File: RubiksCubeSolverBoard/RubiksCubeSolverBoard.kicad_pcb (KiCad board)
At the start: 2 copper layers, 67 x 80.1 mm, 43 parts, among them J1 Power +12V, J10 MS3, J11 MS1, J12 Power +12V, J13 MS2, J14 MS3, J15 Motor2, J16 MS1, J17 MS2, J18 MS3, J19 Motor3, J2 Power +3.3V, J20 MS1, J21 MS2, J22 MS3, J23 Motor4, J24 MS1, J25 MS2, J26 MS3, J27 Motor5, J28 color sensor, J29 color sensor, J3 MS1, J4 BootOption, J6 SilentBoot, J7 Motor1, J8 Uart, J9 MS2, U1 ESP32-WROOM-32E

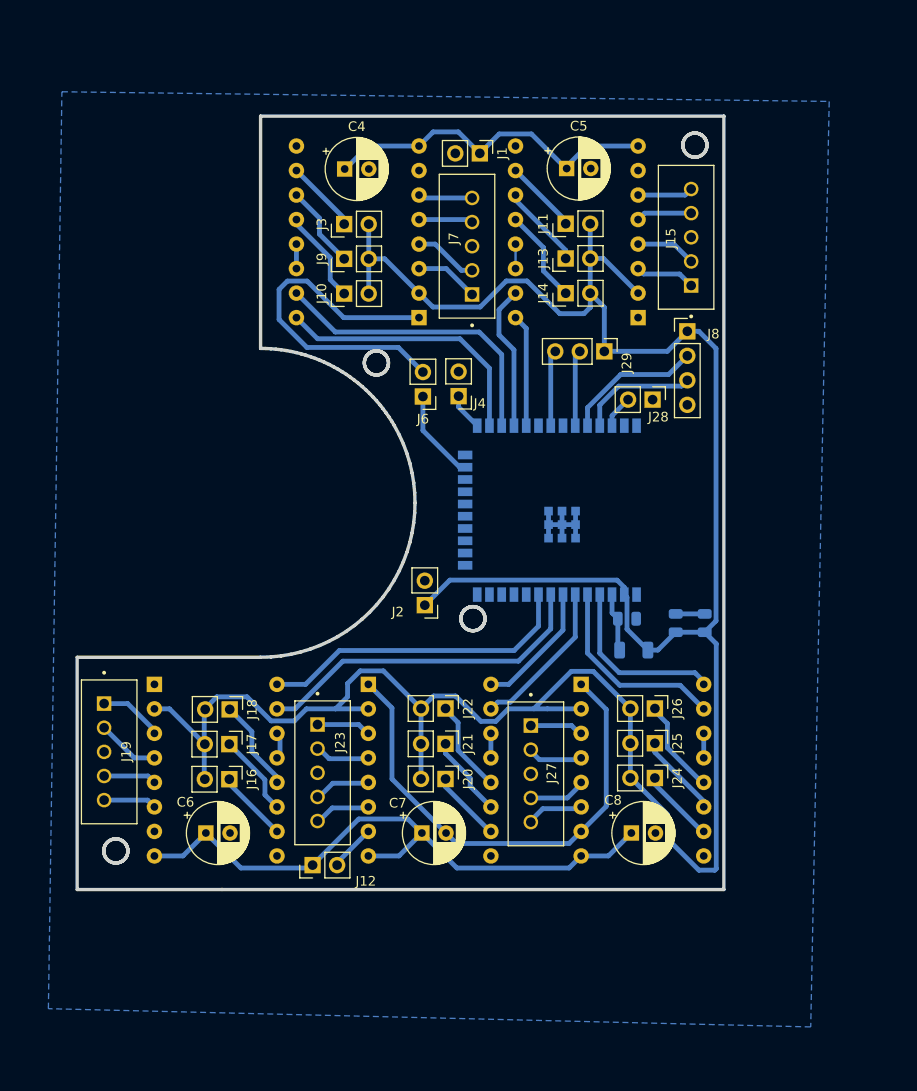
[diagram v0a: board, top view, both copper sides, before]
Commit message: 2 layer pcb
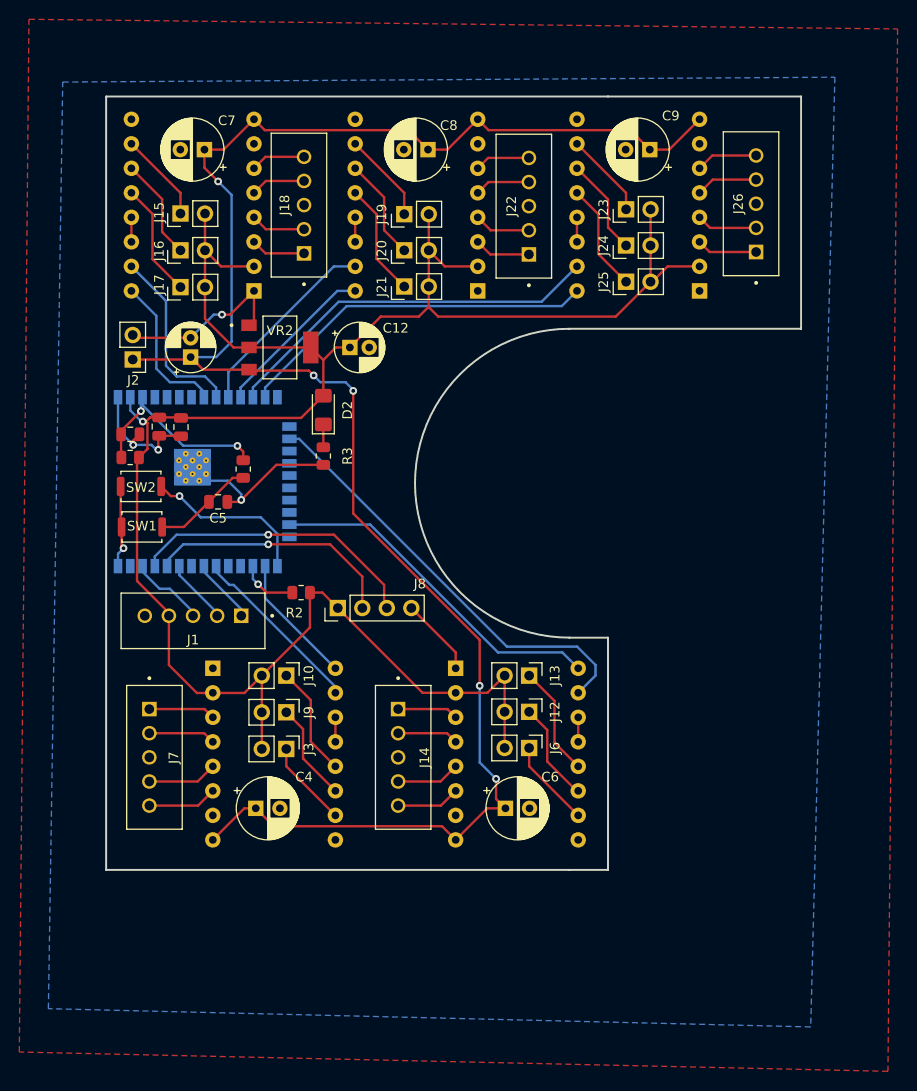
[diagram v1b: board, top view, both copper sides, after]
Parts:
- removed J11: MS1, Connector_PinHeader_2.54mm:PinHeader_1x02_P2.54mm_Vertical
- removed J27: Motor5, CustomParts:JST_B5B-XH-A_LF__SN_
- removed J28: color sensor, Connector_PinHeader_2.54mm:PinHeader_1x02_P2.54mm_Vertical
- removed J29: color sensor, Connector_PinHeader_2.54mm:PinHeader_1x03_P2.54mm_Vertical
- removed J4: BootOption, Connector_PinHeader_2.54mm:PinHeader_1x02_P2.54mm_Vertical
- removed U1: ESP32-WROOM-32E, CustomParts:ESP32-WROOM-32E
- added C11: 10uF, Capacitor_THT:CP_Radial_D5.0mm_P2.00mm, F.Cu at (29.5, 41.8)
- added C12: 10uF, Capacitor_THT:CP_Radial_D5.0mm_P2.00mm, F.Cu at (46.0, 40.8)
- added C9: 100uF, Capacitor_THT:CP_Radial_D6.3mm_P2.50mm, F.Cu at (77.1, 20.3)
- added D2: LED, LED_SMD:LED_1206_3216Metric_Pad1.42x1.75mm_HandSolder, F.Cu at (43.3, 47.3)
- added R2: 10k, Resistor_SMD:R_0805_2012Metric, F.Cu at (41.0, 66.2)
- added R3: 220Ohm, Resistor_SMD:R_0805_2012Metric, F.Cu at (43.3, 52.0)
- added R4: 0, Resistor_SMD:R_0805_2012Metric, F.Cu at (35.0, 53.4)
- added SW1: reset, Button_Switch_SMD:SW_Push_SPST_NO_Alps_SKRK, F.Cu at (24.5, 59.4)
- added SW2: flash, Button_Switch_SMD:SW_Push_SPST_NO_Alps_SKRK, F.Cu at (24.4, 55.2)
- added U2: ESP32-WROOM-32E, RF_Module:ESP32-WROOM-32D, B.Cu at (30.3, 54.7)
- added VR2: TS1117BCW33_RPG, CustomParts:VREG_TS1117BCW33_RPG, F.Cu at (38.8, 40.8)
- C1, C2, C3: moved to F.Cu
- C5: value 100uF -> 0.1uF; footprint Capacitor_THT:CP_Radial_D6.3mm_P2.50mm -> Capacitor_SMD:C_0805_2012Metric
- J1: value Power +12V -> colorSensor; footprint Connector_PinHeader_2.54mm:PinHeader_1x02_P2.54mm_Vertical -> CustomParts:JST_B5B-XH-A_LF__SN_
- J12: value Power +12V -> MS2
- J13, J17, J21, J25: value MS2 -> MS3
- J14: value MS3 -> Motor2; footprint Connector_PinHeader_2.54mm:PinHeader_1x02_P2.54mm_Vertical -> CustomParts:JST_B5B-XH-A_LF__SN_
- J15: value Motor2 -> MS1; footprint CustomParts:JST_B5B-XH-A_LF__SN_ -> Connector_PinHeader_2.54mm:PinHeader_1x02_P2.54mm_Vertical
- J16, J20, J24: value MS1 -> MS2
- J18: value MS3 -> Motor3; footprint Connector_PinHeader_2.54mm:PinHeader_1x02_P2.54mm_Vertical -> CustomParts:JST_B5B-XH-A_LF__SN_
- J19: value Motor3 -> MS1; footprint CustomParts:JST_B5B-XH-A_LF__SN_ -> Connector_PinHeader_2.54mm:PinHeader_1x02_P2.54mm_Vertical
- J2: value Power +3.3V -> power
- J22: value MS3 -> Motor4; footprint Connector_PinHeader_2.54mm:PinHeader_1x02_P2.54mm_Vertical -> CustomParts:JST_B5B-XH-A_LF__SN_
- J23: value Motor4 -> MS1; footprint CustomParts:JST_B5B-XH-A_LF__SN_ -> Connector_PinHeader_2.54mm:PinHeader_1x02_P2.54mm_Vertical
- J26: value MS3 -> Motor5; footprint Connector_PinHeader_2.54mm:PinHeader_1x02_P2.54mm_Vertical -> CustomParts:JST_B5B-XH-A_LF__SN_
- J6: value SilentBoot -> MS1
- R1: footprint Resistor_SMD:R_1206_3216Metric -> Resistor_SMD:R_0805_2012Metric; moved to F.Cu
- moved C7 74.3 mm to (31.0, 20.3), turned to 180 degrees
- moved C8 73.9 mm to (54.1, 20.3), turned to 180 degrees
- moved C4 66.9 mm to (36.3, 88.5)
- moved J23 66.3 mm to (74.7, 26.5), turned to 90 degrees
- moved J19 63.5 mm to (51.7, 27.0), turned to 90 degrees
- moved J7 62.1 mm to (25.8, 83.3), turned to -90 degrees
- moved C1 57.9 mm to (28.5, 49.0), turned to -90 degrees
- moved C2 57.3 mm to (26.3, 49.0), turned to -90 degrees
- moved J1 56.8 mm to (29.8, 69.1), turned to 180 degrees
- moved R1 55.9 mm to (23.3, 52.2)
- moved J24 55.3 mm to (74.7, 30.2), turned to 90 degrees
- moved J16 55.0 mm to (28.5, 30.7), turned to 90 degrees
- moved J20 54.9 mm to (51.7, 30.7), turned to 90 degrees
- moved C3 54.9 mm to (23.3, 49.8)
- moved J3 54.7 mm to (39.5, 82.4), turned to -90 degrees
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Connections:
- net Net-(U1-EN) renamed EN
- A1 pad 15: IO16 -> motor1Step
- A1 pad 16: IO4 -> motor1Dir
- A2 pad 15: IO17 -> motor2Step
- A2 pad 16: IO5 -> motor2Dir
- A3 pad 15: IO32 -> motor3Step
- A3 pad 16: IO33 -> motor3Dir
- A4 pad 15: IO34 -> motor4Step
- A4 pad 16: IO35 -> motor4Dir
- A5 pad 15: IO39 -> motor5Step
- A5 pad 16: IO36 -> motor5Dir
- C5 pad 1: +12V -> GND
- C5 pad 2: GND -> Net-(C5-Pad2)
- J1 pad 1: +12V -> colorSensorLed
- J1 pad 2: GND -> SDA
- J12 pad 1: +12V -> Net-(A2-MS2)
- J12 pad 2: GND -> +3.3V
- J13 pad 1: Net-(A2-MS2) -> Net-(A2-MS3)
- J14 pad 1: Net-(A2-MS3) -> Net-(A2-1B)
- J14 pad 2: +3.3V -> Net-(A2-1A)
- J15 pad 1: Net-(A2-1B) -> Net-(A3-MS1)
- J15 pad 2: Net-(A2-1A) -> +3.3V
- J16 pad 1: Net-(A3-MS1) -> Net-(A3-MS2)
- J17 pad 1: Net-(A3-MS2) -> Net-(A3-MS3)
- J18 pad 1: Net-(A3-MS3) -> Net-(A3-1B)
- J18 pad 2: +3.3V -> Net-(A3-1A)
- J19 pad 1: Net-(A3-1B) -> Net-(A4-MS1)
- J19 pad 2: Net-(A3-1A) -> +3.3V
- J2 pad 1: +3.3V -> +12V
- J20 pad 1: Net-(A4-MS1) -> Net-(A4-MS2)
- J21 pad 1: Net-(A4-MS2) -> Net-(A4-MS3)
- J22 pad 1: Net-(A4-MS3) -> Net-(A4-1B)
- J22 pad 2: +3.3V -> Net-(A4-1A)
- J23 pad 1: Net-(A4-1B) -> Net-(A5-MS1)
- J23 pad 2: Net-(A4-1A) -> +3.3V
- J24 pad 1: Net-(A5-MS1) -> Net-(A5-MS2)
- J25 pad 1: Net-(A5-MS2) -> Net-(A5-MS3)
- J26 pad 1: Net-(A5-MS3) -> Net-(A5-1B)
- J26 pad 2: +3.3V -> Net-(A5-1A)
- J6 pad 1: Net-(J6-Pin_1) -> Net-(A2-MS1)
- J6 pad 2: GND -> +3.3V
- J8 pad 2: Net-(J8-Pin_2) -> RX
- J8 pad 3: Net-(J8-Pin_3) -> TX
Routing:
- net +12V: track 100.1 -> 192.4 mm, vias 0 -> 5
- net +3.3V: track 267.7 -> 214.0 mm, vias 0 -> 1
- net motor2Step: track 0.00 -> 45.0 mm
- net motor5Step: track 0.00 -> 39.8 mm
- net motor5Dir: track 0.00 -> 37.5 mm
- net motor2Dir: track 0.00 -> 36.1 mm
- net IO32: track 35.0 -> 0.00 mm
- net IO33: track 32.5 -> 0.00 mm
- net IO16: track 31.3 -> 0.00 mm
- net TX: track 0.00 -> 30.4 mm, vias 0 -> 1
- net GND: track 95.6 -> 66.1 mm, vias 0 -> 5
- net IO4: track 28.1 -> 0.00 mm
- net RX: track 0.00 -> 26.1 mm, vias 0 -> 1
- net IO39: track 20.5 -> 0.00 mm
- net motor4Step: track 0.00 -> 20.3 mm
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- added copper zone on F.Cu, net GND
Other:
- board size 67 x 80.1 mm -> 72 x 80.1 mm
